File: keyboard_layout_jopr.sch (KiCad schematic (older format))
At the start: 229 parts, among them SW1 SW_Push, U1 ATmega32U4-AU, U2 TPD4EUSB30, Y1 16MHz

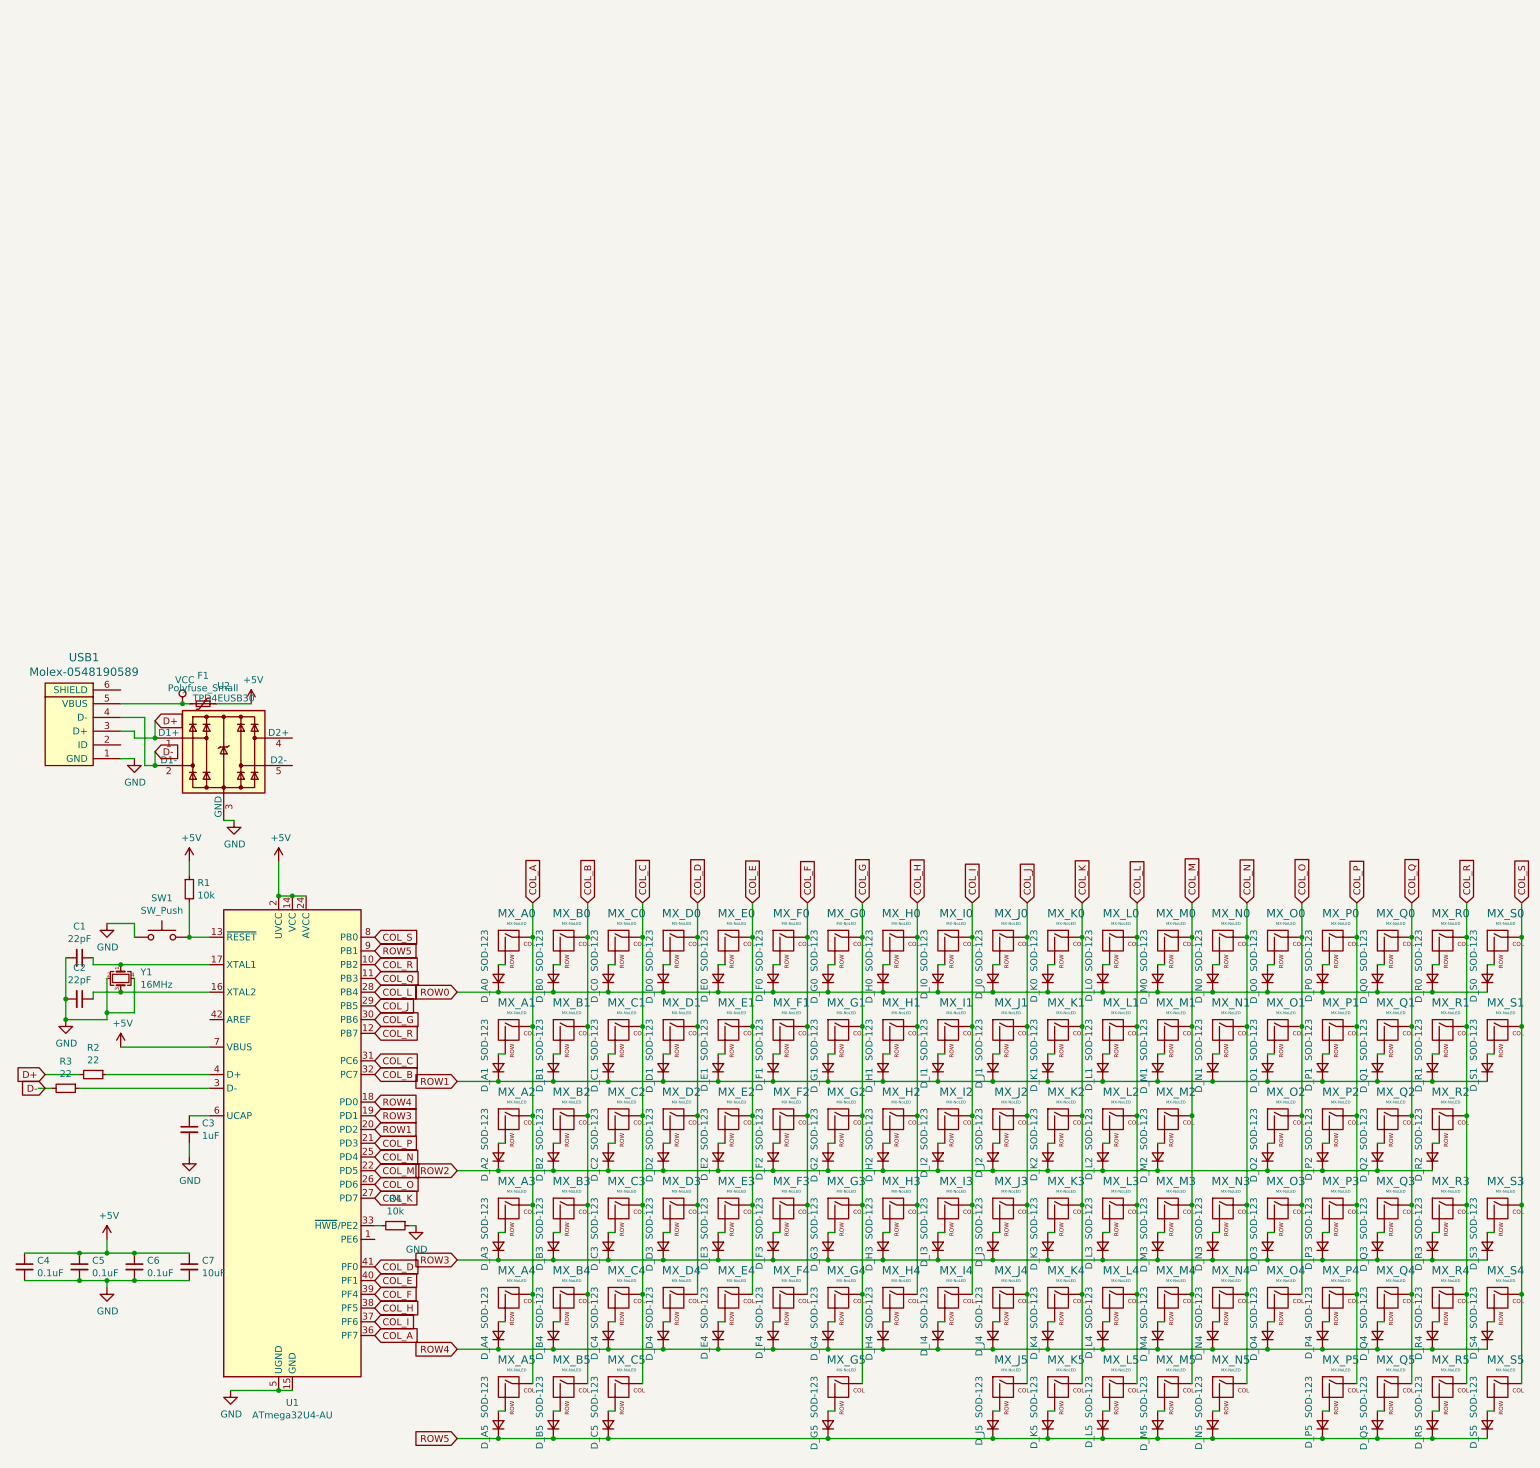
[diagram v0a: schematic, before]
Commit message: squared matrix, updated and renamed PDFs
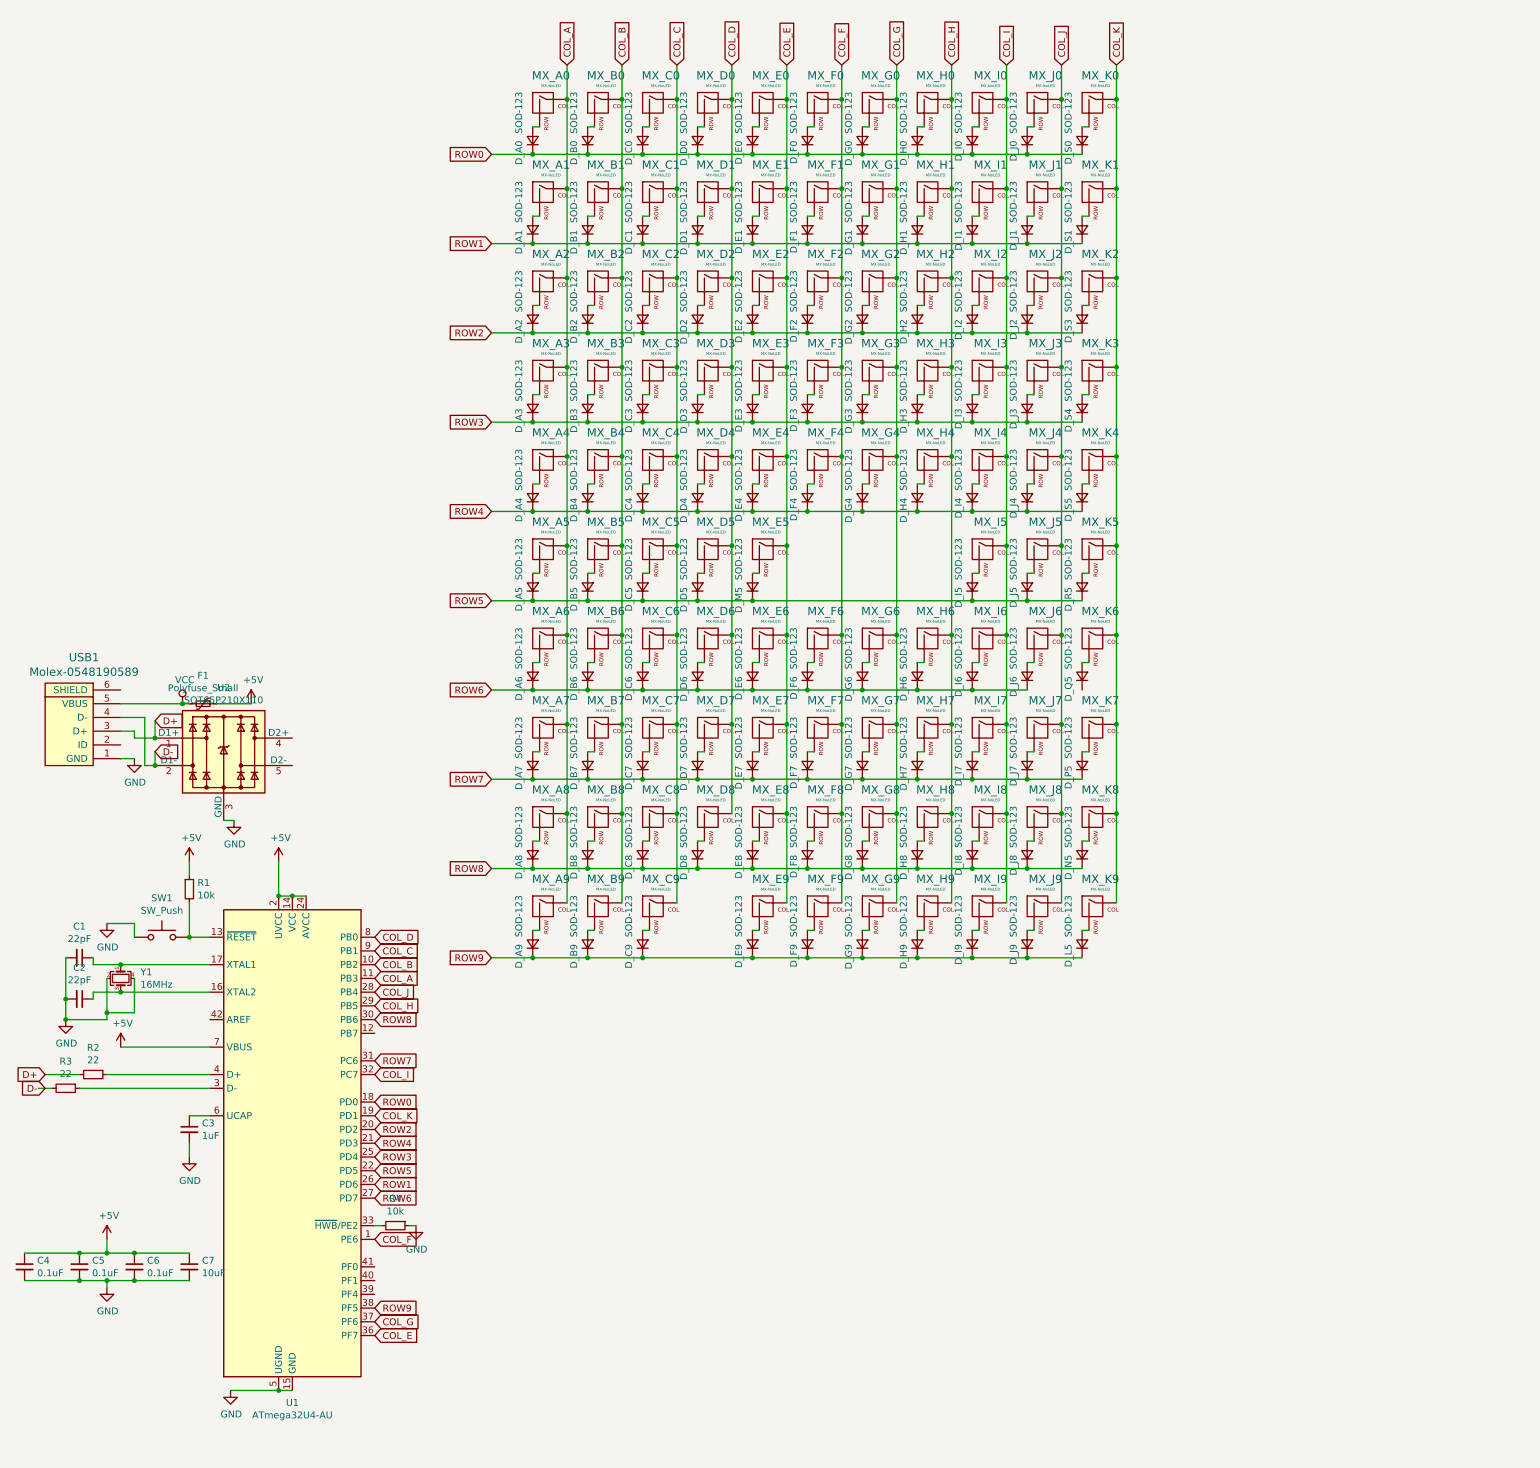
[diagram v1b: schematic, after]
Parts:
- removed U2: TPD4EUSB30, SOT65P210X110-6N:SOT65P210X110-6N, symbol Power_Protection:TPD4EUSB30
- added U2: SOT65P210X110, SOT65P210X110-6N:SOT65P210X110-6N, symbol Power_Protection:SOT65P210X110
- renumbered D_K0 to D_A6, D_K1 to D_A7, D_K2 to D_A8, D_K3 to D_A9, D_L0 to D_B6, D_L1 to D_B7, D_L2 to D_B8, D_L3 to D_B9, D_M0 to D_C6, D_M1 to D_C7, D_M2 to D_C8, D_M3 to D_C9, D_G5 to D_D5, D_N0 to D_D6, D_N1 to D_D7, D_N3 to D_D8, D_O0 to D_E6, D_O1 to D_E7, D_O2 to D_E8, D_O3 to D_E9, D_P0 to D_F6, D_P1 to D_F7, D_P2 to D_F8, D_P3 to D_F9, D_Q0 to D_G6, D_Q1 to D_G7, D_Q2 to D_G8, D_Q3 to D_G9, D_R0 to D_H6, D_R1 to D_H7, D_R2 to D_H8, D_R3 to D_H9, D_K5 to D_I5, D_N4 to D_I6, D_M4 to D_I7, D_L4 to D_I8, D_K4 to D_I9, D_R4 to D_J6, D_Q4 to D_J7, D_P4 to D_J8, D_O4 to D_J9, MX_K0 to MX_A6, MX_K1 to MX_A7, MX_K2 to MX_A8, MX_K3 to MX_A9, MX_L0 to MX_B6, MX_L1 to MX_B7, MX_L2 to MX_B8, MX_L3 to MX_B9, MX_M0 to MX_C6, MX_M1 to MX_C7, MX_M2 to MX_C8, MX_M3 to MX_C9, MX_G5 to MX_D5, MX_N0 to MX_D6, MX_N1 to MX_D7, MX_N3 to MX_D8, MX_M5 to MX_E5, MX_O0 to MX_E6, MX_O1 to MX_E7, MX_O2 to MX_E8, MX_O3 to MX_E9, MX_P0 to MX_F6, MX_P1 to MX_F7, MX_P2 to MX_F8, MX_P3 to MX_F9, MX_Q0 to MX_G6, MX_Q1 to MX_G7, MX_Q2 to MX_G8, MX_Q3 to MX_G9, MX_R0 to MX_H6, MX_R1 to MX_H7, MX_R2 to MX_H8, MX_R3 to MX_H9, MX_K5 to MX_I5, MX_N4 to MX_I6, MX_M4 to MX_I7, MX_L4 to MX_I8, MX_K4 to MX_I9, MX_R4 to MX_J6, MX_Q4 to MX_J7, MX_P4 to MX_J8, MX_O4 to MX_J9, MX_S0 to MX_K0, MX_S1 to MX_K1, MX_S3 to MX_K2, MX_S4 to MX_K3, MX_S5 to MX_K4, MX_R5 to MX_K5, MX_Q5 to MX_K6, MX_P5 to MX_K7, MX_N5 to MX_K8, MX_L5 to MX_K9
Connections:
- net COL_A: now also MX_A6.1 (COL), MX_A7.1 (COL), MX_A8.1 (COL), MX_A9.1 (COL), U1.11 (PB3); no longer U1.36 (PF7)
- net COL_B: now also MX_B6.1 (COL), MX_B7.1 (COL), MX_B8.1 (COL), MX_B9.1 (COL), U1.10 (PB2); no longer U1.32 (PC7)
- net COL_C: now also MX_C6.1 (COL), MX_C7.1 (COL), MX_C8.1 (COL), MX_C9.1 (COL), U1.9 (PB1); no longer U1.31 (PC6)
- net COL_D: now also MX_D5.1 (COL), MX_D6.1 (COL), MX_D7.1 (COL), MX_D8.1 (COL), U1.8 (PB0); no longer U1.41 (PF0)
- net COL_E: now also MX_E5.1 (COL), MX_E6.1 (COL), MX_E7.1 (COL), MX_E8.1 (COL), MX_E9.1 (COL), U1.36 (PF7); no longer U1.40 (PF1)
- net COL_F: now also MX_F6.1 (COL), MX_F7.1 (COL), MX_F8.1 (COL), MX_F9.1 (COL), U1.1 (PE6); no longer U1.39 (PF4)
- net COL_G: now also MX_G6.1 (COL), MX_G7.1 (COL), MX_G8.1 (COL), MX_G9.1 (COL), U1.37 (PF6); no longer MX_D5.1 (COL), U1.30 (PB6)
- net COL_H: now also MX_H6.1 (COL), MX_H7.1 (COL), MX_H8.1 (COL), MX_H9.1 (COL), U1.29 (PB5); no longer U1.38 (PF5)
- net COL_I: now also MX_I5.1 (COL), MX_I6.1 (COL), MX_I7.1 (COL), MX_I8.1 (COL), MX_I9.1 (COL), U1.32 (PC7); no longer U1.37 (PF6)
- net COL_J: now also MX_J6.1 (COL), MX_J7.1 (COL), MX_J8.1 (COL), MX_J9.1 (COL), U1.28 (PB4); no longer U1.29 (PB5)
- net COL_K: now also MX_K0.1 (COL), MX_K1.1 (COL), MX_K2.1 (COL), MX_K3.1 (COL), MX_K4.1 (COL), MX_K5.1 (COL), MX_K6.1 (COL), MX_K7.1 (COL), MX_K8.1 (COL), MX_K9.1 (COL), U1.19 (PD1); no longer MX_A6.1 (COL), MX_A7.1 (COL), MX_A8.1 (COL), MX_A9.1 (COL), MX_I5.1 (COL), MX_I9.1 (COL), U1.27 (PD7)
- net D+: now also U2.1 (D1+)
- net D-: now also U2.2 (D1-)
- net GND: now also U2.3 (GND), U2.8 (GND)
- net ROW0: now also U1.18 (PD0); no longer D_A6.1 (K), D_B6.1 (K), D_C6.1 (K), D_D6.1 (K), D_E6.1 (K), D_F6.1 (K), D_G6.1 (K), D_H6.1 (K)
- net ROW1: now also U1.26 (PD6); no longer D_A7.1 (K), D_B7.1 (K), D_C7.1 (K), D_D7.1 (K), D_E7.1 (K), D_F7.1 (K), D_G7.1 (K), D_H7.1 (K), U1.20 (PD2)
- net ROW2: now also D_S3.1 (K), U1.20 (PD2); no longer D_A8.1 (K), D_B8.1 (K), D_C8.1 (K), D_E8.1 (K), D_F8.1 (K), D_G8.1 (K), D_H8.1 (K)
- net ROW3: now also D_S4.1 (K), U1.25 (PD4); no longer D_A9.1 (K), D_B9.1 (K), D_C9.1 (K), D_D8.1 (K), D_E9.1 (K), D_F9.1 (K), D_G9.1 (K), D_H9.1 (K), D_S3.1 (K), U1.19 (PD1)
- net ROW4: now also D_S5.1 (K), U1.21 (PD3); no longer D_I6.1 (K), D_I7.1 (K), D_I8.1 (K), D_I9.1 (K), D_J6.1 (K), D_J7.1 (K), D_J8.1 (K), D_J9.1 (K), D_S4.1 (K), U1.18 (PD0)
- net ROW5: now also U1.22 (PD5); no longer D_L5.1 (K), D_N5.1 (K), D_P5.1 (K), D_Q5.1 (K), D_S5.1 (K), U1.9 (PB1)
- removed net COL_L: MX_B6.1 (COL), MX_B7.1 (COL), MX_B8.1 (COL), MX_B9.1 (COL), MX_I8.1 (COL), MX_K9.1 (COL), U1.28 (PB4)
- removed net COL_M: MX_C6.1 (COL), MX_C7.1 (COL), MX_C8.1 (COL), MX_C9.1 (COL), MX_E5.1 (COL), MX_I7.1 (COL), U1.22 (PD5)
- removed net COL_N: MX_D6.1 (COL), MX_D7.1 (COL), MX_D8.1 (COL), MX_I6.1 (COL), MX_K8.1 (COL), U1.25 (PD4)
- removed net COL_O: MX_E6.1 (COL), MX_E7.1 (COL), MX_E8.1 (COL), MX_E9.1 (COL), MX_J9.1 (COL), U1.26 (PD6)
- removed net COL_P: MX_F6.1 (COL), MX_F7.1 (COL), MX_F8.1 (COL), MX_F9.1 (COL), MX_J8.1 (COL), MX_K7.1 (COL), U1.21 (PD3)
- removed net COL_Q: MX_G6.1 (COL), MX_G7.1 (COL), MX_G8.1 (COL), MX_G9.1 (COL), MX_J7.1 (COL), MX_K6.1 (COL), U1.11 (PB3)
- removed net COL_R: MX_H6.1 (COL), MX_H7.1 (COL), MX_H8.1 (COL), MX_H9.1 (COL), MX_J6.1 (COL), MX_K5.1 (COL), U1.10 (PB2), U1.12 (PB7)
- removed net COL_S: MX_K0.1 (COL), MX_K1.1 (COL), MX_K2.1 (COL), MX_K3.1 (COL), MX_K4.1 (COL), U1.8 (PB0)
- new net ROW6: D_A6.1 (K), D_B6.1 (K), D_C6.1 (K), D_D6.1 (K), D_E6.1 (K), D_F6.1 (K), D_G6.1 (K), D_H6.1 (K), D_I6.1 (K), D_J6.1 (K), U1.27 (PD7)
- new net ROW7: D_A7.1 (K), D_B7.1 (K), D_C7.1 (K), D_D7.1 (K), D_E7.1 (K), D_F7.1 (K), D_G7.1 (K), D_H7.1 (K), D_I7.1 (K), D_J7.1 (K), D_P5.1 (K), U1.31 (PC6)
- new net ROW8: D_A8.1 (K), D_B8.1 (K), D_C8.1 (K), D_D8.1 (K), D_E8.1 (K), D_F8.1 (K), D_G8.1 (K), D_H8.1 (K), D_I8.1 (K), D_J8.1 (K), D_N5.1 (K), U1.30 (PB6)
- new net ROW9: D_A9.1 (K), D_B9.1 (K), D_C9.1 (K), D_E9.1 (K), D_F9.1 (K), D_G9.1 (K), D_H9.1 (K), D_I9.1 (K), D_J9.1 (K), D_L5.1 (K), U1.38 (PF5)
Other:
- moved on the sheet: D_A0, D_A1, D_A2, D_A3, D_A4, D_A5, D_A6, D_A7, D_A8, D_A9, D_B0, D_B1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
